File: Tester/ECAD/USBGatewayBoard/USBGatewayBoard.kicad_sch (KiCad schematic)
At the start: 5 parts, among them J1 Conn_02x20_Odd_Even

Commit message: Progressed ECAD
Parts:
- J1: Manufacturer Part Number https://datasheet.lcsc.com/lcsc/1810311440_Nextron-Nextroni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 -> Z-231011020106
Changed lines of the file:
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@@
       (effects (font (size 1.27 1.27)) hide)
     )
-    (property "Datasheet" "Z-231011020106" (id 3) (at 227.33 96.52 0)
-      (effects (font (size 1.27 1.27)) hide)
-    )
-    (property "Manufacturer Part Number" "https://datasheet.lcsc.com/lcsc/1810311440_Nextron-Nextronics-Engineering-Z-231011020106_C221051.pdf" (id 4) (at 227.33 96.52 0)
+    (property "Datasheet" "https://datasheet.lcsc.com/lcsc/1810311440_Nextron-Nextronics-Engineering-Z-231011020106_C221051.pdf" (id 3) (at 227.33 96.52 0)
+      (effects (font (size 1.27 1.27)) hide)
+    )
+    (property "Manufacturer Part Number" "Z-231011020106" (id 4) (at 227.33 96.52 0)
       (effects (font (size 1.27 1.27)) hide)
     )
@@
       (reference "R28") (unit 1) (value "R") (footprint "Resistor_SMD:R_0805_2012Metric_Pad1.20x1.40mm_HandSolder")
     )
+    (path "/76be5f40-0efd-4be0-a528-34098d56af2b/50fcc21e-e085-4943-9a28-8f39c2cf0805"
+      (reference "U1") (unit 1) (value "ATSAMD21G18A-A") (footprint "Package_QFP:TQFP-48_7x7mm_P0.5mm")
+    )
     (path "/897e9868-1ae5-45cd-ab61-45d0dcbc33eb/22d82e24-0696-4dab-a97d-f101260ef0aa"

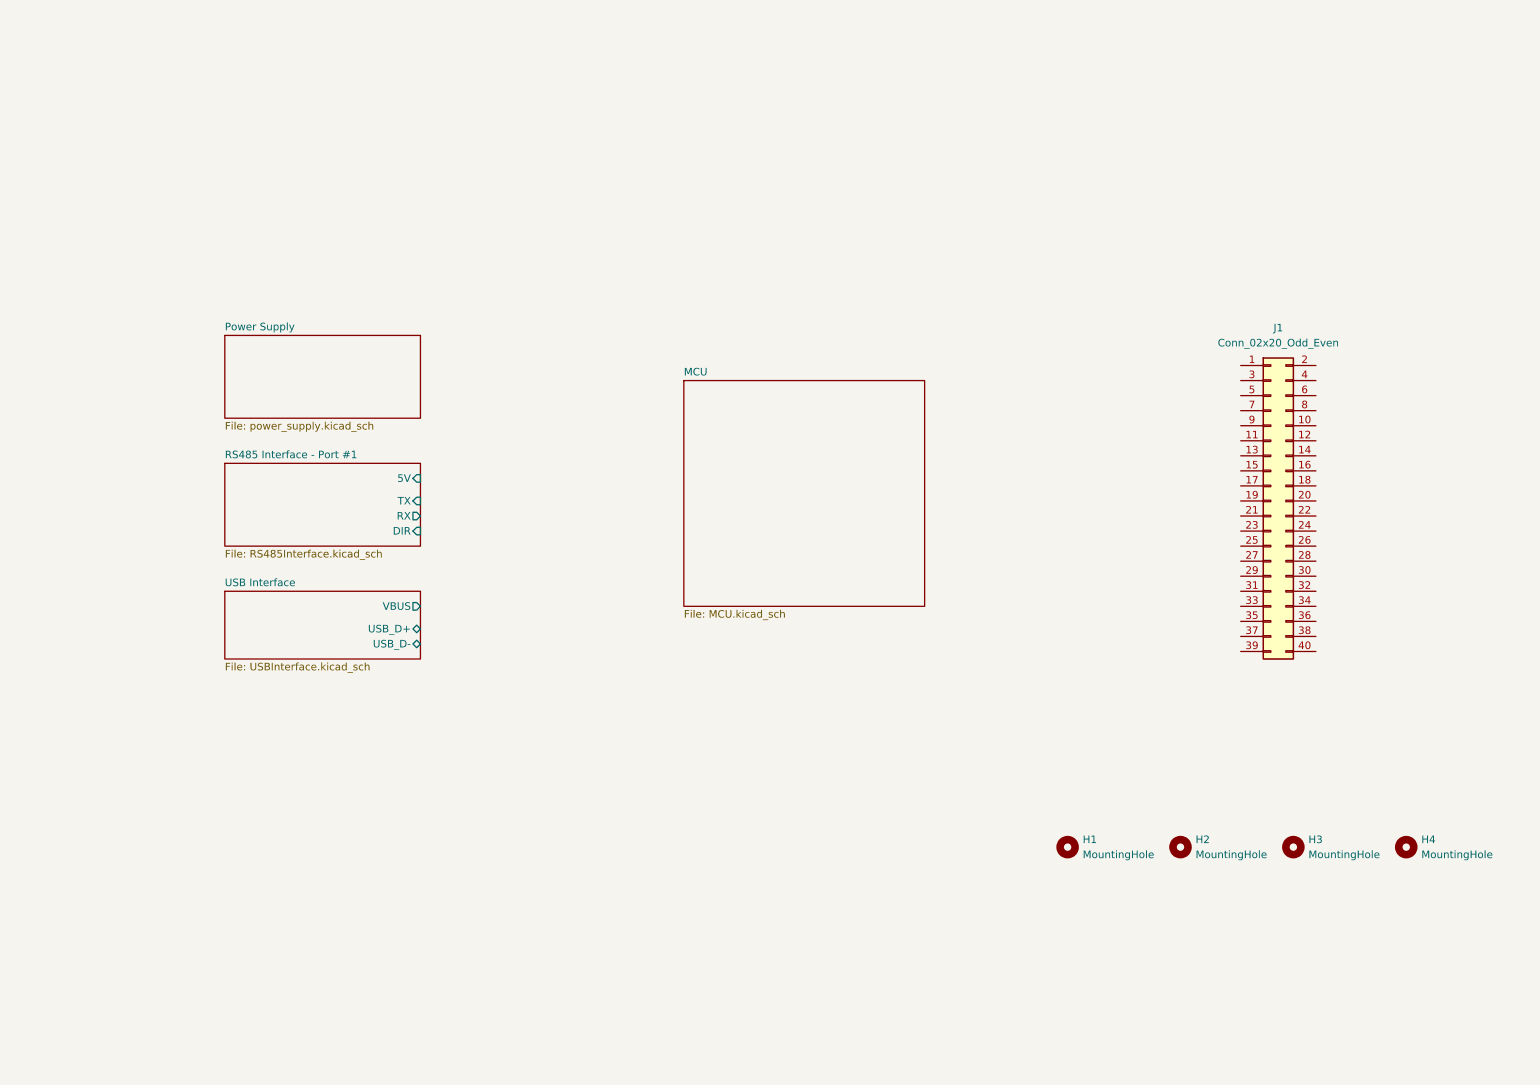
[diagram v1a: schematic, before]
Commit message: Progressed ECAD
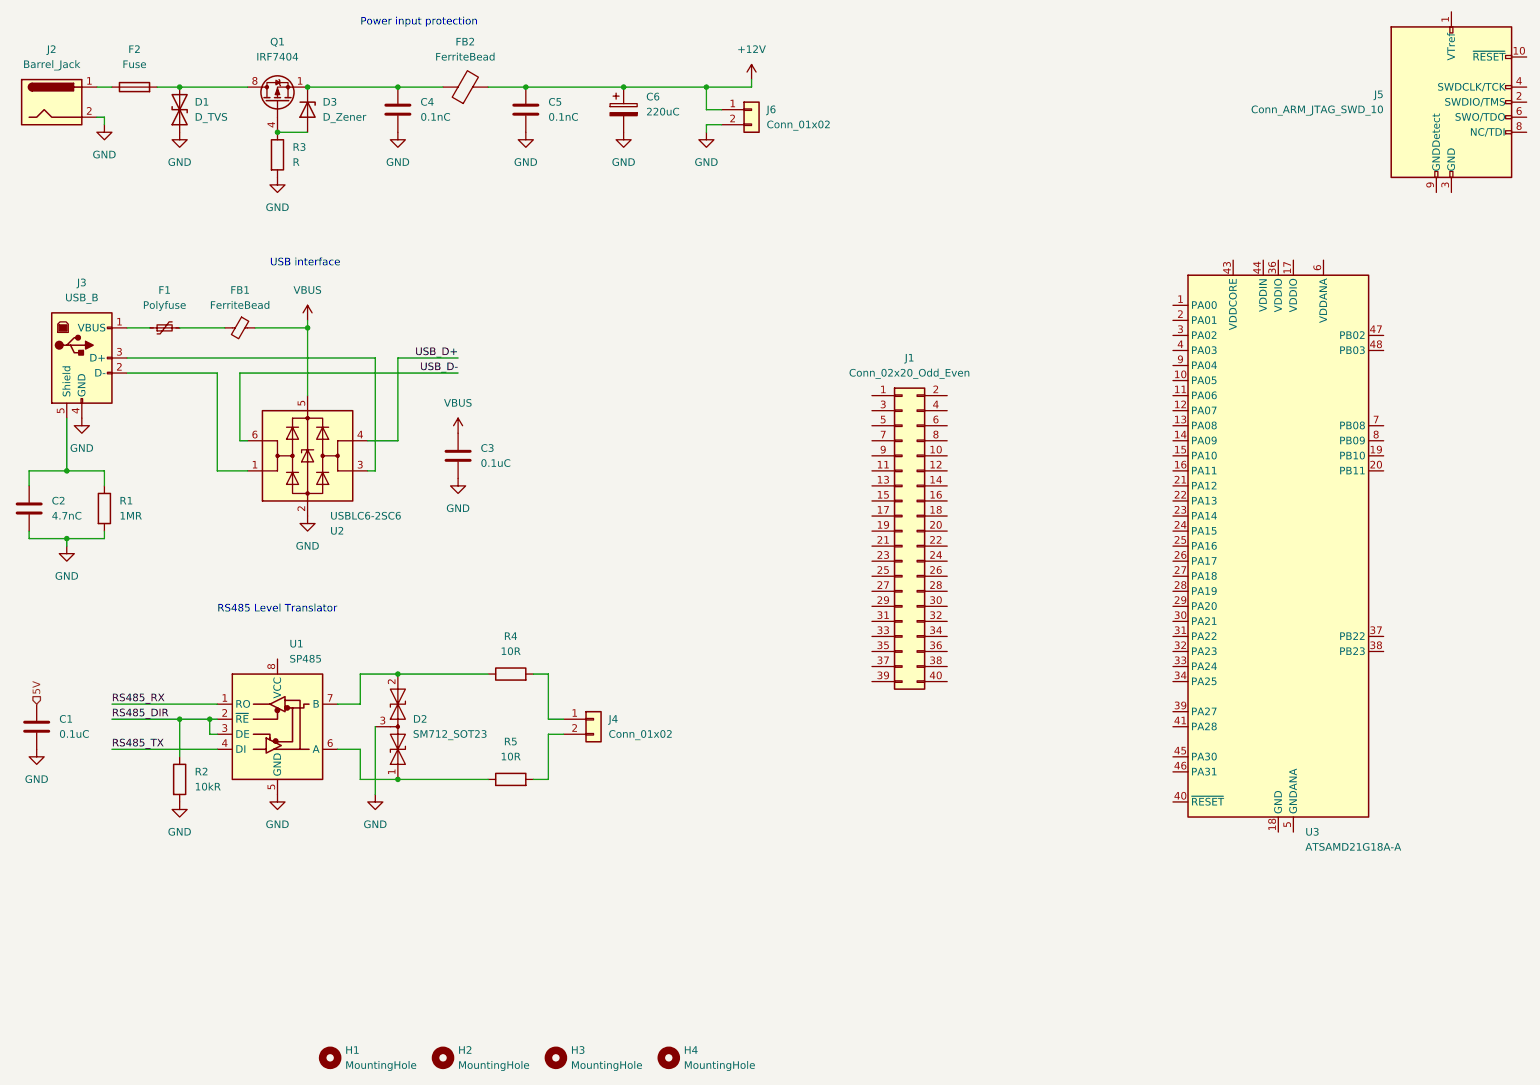
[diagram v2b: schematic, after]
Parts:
- added C1, C3: 0.1uC, Capacitor_SMD:C_0805_2012Metric_Pad1.18x1.45mm_HandSolder, symbol Device:C
- added C2: 4.7nC, Capacitor_SMD:C_0805_2012Metric_Pad1.18x1.45mm_HandSolder, symbol Device:C
- added C4, C5: 0.1nC, Capacitor_SMD:C_0805_2012Metric_Pad1.18x1.45mm_HandSolder, symbol Device:C
- added C6: 220uC, Capacitor_THT:CP_Radial_D8.0mm_P3.50mm, symbol Device:C_Polarized
- added D1: D_TVS, Diode_SMD:D_SMA, symbol Device:D_TVS
- added D2: SM712_SOT23, Package_TO_SOT_SMD:SOT-23, symbol Diode:SM712_SOT23
- added D3: D_Zener, symbol Device:D_Zener
- added F1: Polyfuse, Fuse:Fuse_0805_2012Metric_Pad1.15x1.40mm_HandSolder, symbol Device:Polyfuse_Small
- added F2: Fuse, symbol Device:Fuse
- added FB1: FerriteBead, Inductor_SMD:L_0805_2012Metric_Pad1.15x1.40mm_HandSolder, symbol Device:FerriteBead_Small
- added FB2: FerriteBead, Inductor_SMD:L_1806_4516Metric_Pad1.45x1.90mm_HandSolder, symbol Device:FerriteBead
- added J2: Barrel_Jack, symbol Connector:Barrel_Jack
- added J3: USB_B, Connector_USB:USB_B_OST_USB-B1HSxx_Horizontal, symbol Connector:USB_B
- added J4, J6: Conn_01x02, symbol Connector_Generic:Conn_01x02
- added J5: Conn_ARM_JTAG_SWD_10, symbol Connector:Conn_ARM_JTAG_SWD_10
- added Q1: IRF7404, Package_SO:SOIC-8_3.9x4.9mm_P1.27mm, symbol Transistor_FET:IRF7404
- added R1: 1MR, Resistor_SMD:R_0805_2012Metric_Pad1.20x1.40mm_HandSolder, symbol Device:R
- added R2: 10kR, Resistor_SMD:R_0805_2012Metric_Pad1.20x1.40mm_HandSolder, symbol Device:R
- added R3: R, Resistor_SMD:R_0805_2012Metric_Pad1.20x1.40mm_HandSolder, symbol Device:R
- added R4, R5: 10R, Resistor_SMD:R_0805_2012Metric_Pad1.20x1.40mm_HandSolder, symbol Device:R
- added U1: SP485, Package_SO:SOIC-8_3.9x4.9mm_P1.27mm, symbol Interface_UART:ST485EBDR
- added U2: USBLC6-2SC6, Package_TO_SOT_SMD:SOT-23-6, symbol Power_Protection:USBLC6-2SC6
- added U3: ATSAMD21G18A-A, Package_QFP:TQFP-48_7x7mm_P0.5mm, symbol MCU_Microchip_SAMD:ATSAMD21G18A-A
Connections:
- new net: C4.1, D3.1 (K), FB2.1, Q1.1 (S), Q1.2 (S), Q1.3 (S)
- new net: D3.2 (A), Q1.4 (G), R3.1
- new net: D1.2 (A2), F2.2, Q1.5 (D), Q1.6 (D), Q1.7 (D), Q1.8 (D)
- new net: F2.1, J2.1
- new net: F1.1, J3.1 (VBUS)
- new net: J3.2 (D-), U2.1 (I/O1)
- new net: J3.3 (D+), U2.3 (I/O2)
- new net: C2.1, J3.5 (Shield), R1.1
- new net: D2.1 (A1), R5.1, U1.6 (A)
- new net: D2.2 (A2), R4.1, U1.7 (B)
- new net: J5.3 (GND), J5.5 (GND)
- new net: J4.1 (Pin_1), R4.2
- new net: J4.2 (Pin_2), R5.2
- new net: F1.2, FB1.2
- new net: U3.18 (GND), U3.35 (GND), U3.42 (GND)
- new net +12V: C5.1, C6.1, FB2.2, J6.1 (Pin_1)
- new net 5V: C1.2
- new net GND: C1.1, C2.2, C3.1, C4.2, C5.2, C6.2, D1.1 (A1), D2.3 (common), J2.2, J3.4 (GND), J6.2 (Pin_2), R1.2, R2.2, R3.2, U1.5 (GND), U2.2 (GND)
- new net RS485_DIR: R2.1, U1.2 (~{RE}), U1.3 (DE)
- new net RS485_RX: U1.1 (RO)
- new net RS485_TX: U1.4 (DI)
- new net USB_D+: U2.4 (I/O2)
- new net USB_D-: U2.6 (I/O1)
- new net VBUS: C3.2, FB1.1, U2.5 (VBUS)
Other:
- removed sheet MCU
- removed sheet Power Supply
- removed sheet RS485 Interface - Port #1
- removed sheet USB Interface
- note added: "Power input protection"
- note added: "RS485 Level Translator"
- note added: "USB interface"
- moved on the sheet: H1, H2, H3, H4, J1
